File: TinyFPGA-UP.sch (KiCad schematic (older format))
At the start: 35 parts, among them J1 Conn_01x14, J2 Conn_01x14, J3 USB_B_Micro, J4 Conn_02x08_Odd_Even, J5 Conn_02x03_Odd_Even, SW1 SW_Push, U1 iCE40-UP5K-SG48, U2 MIC5504-3.3, U3 DSC6001CI2A, U4 MIC5365-1.2, U5 AT25SF081

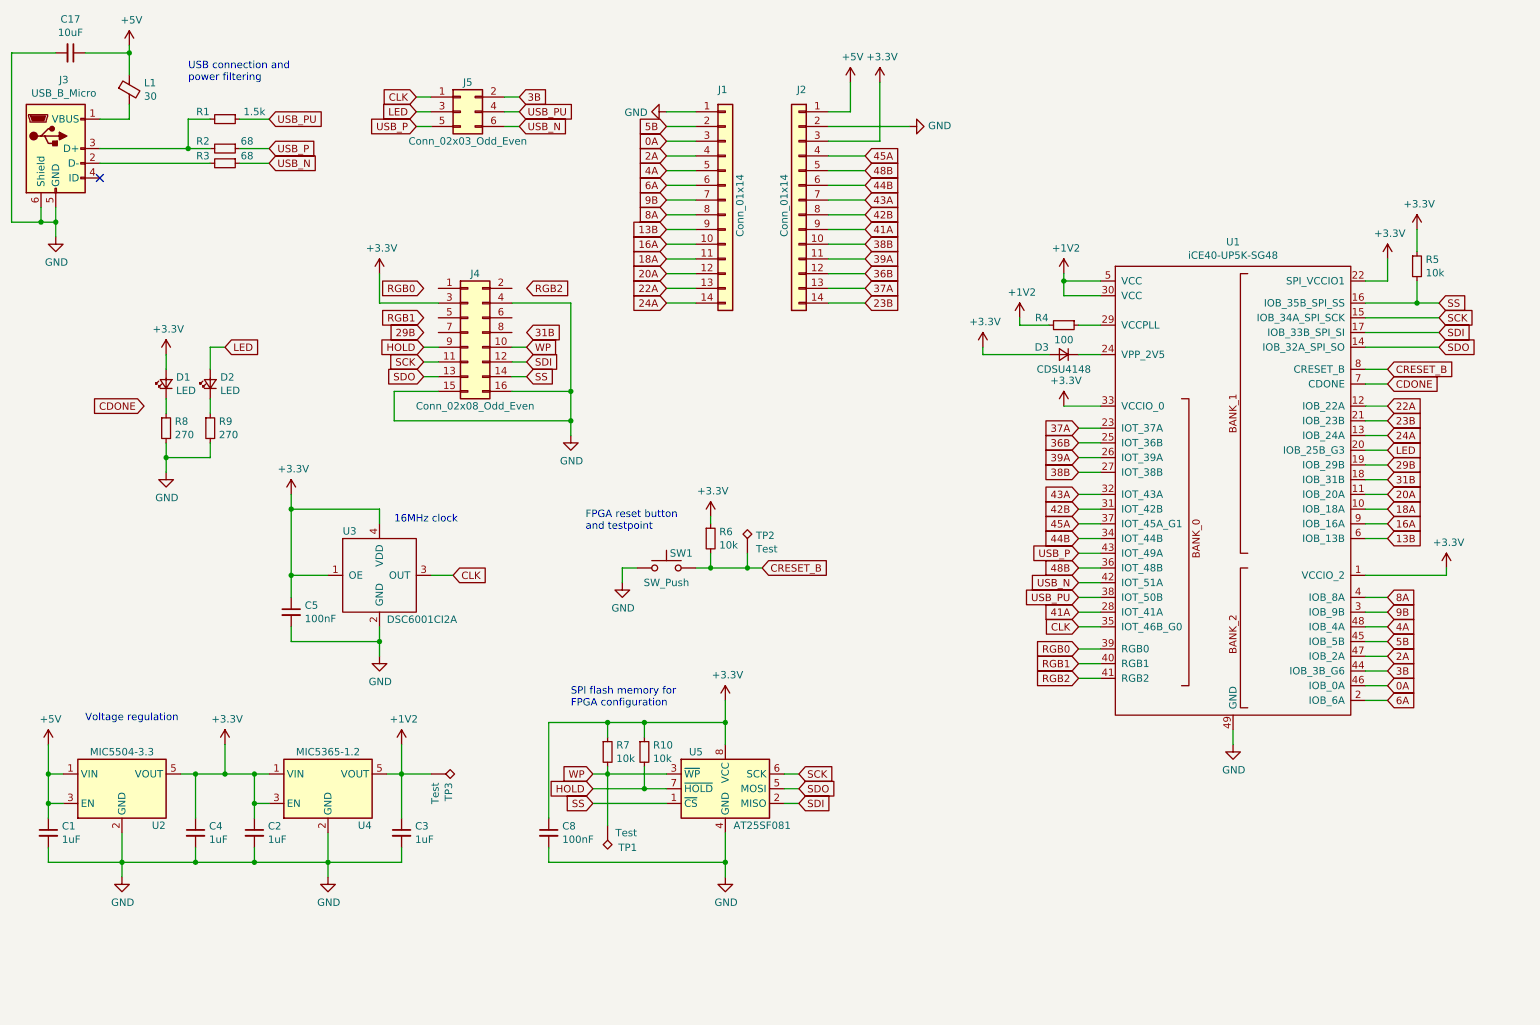
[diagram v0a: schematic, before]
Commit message: Update routing
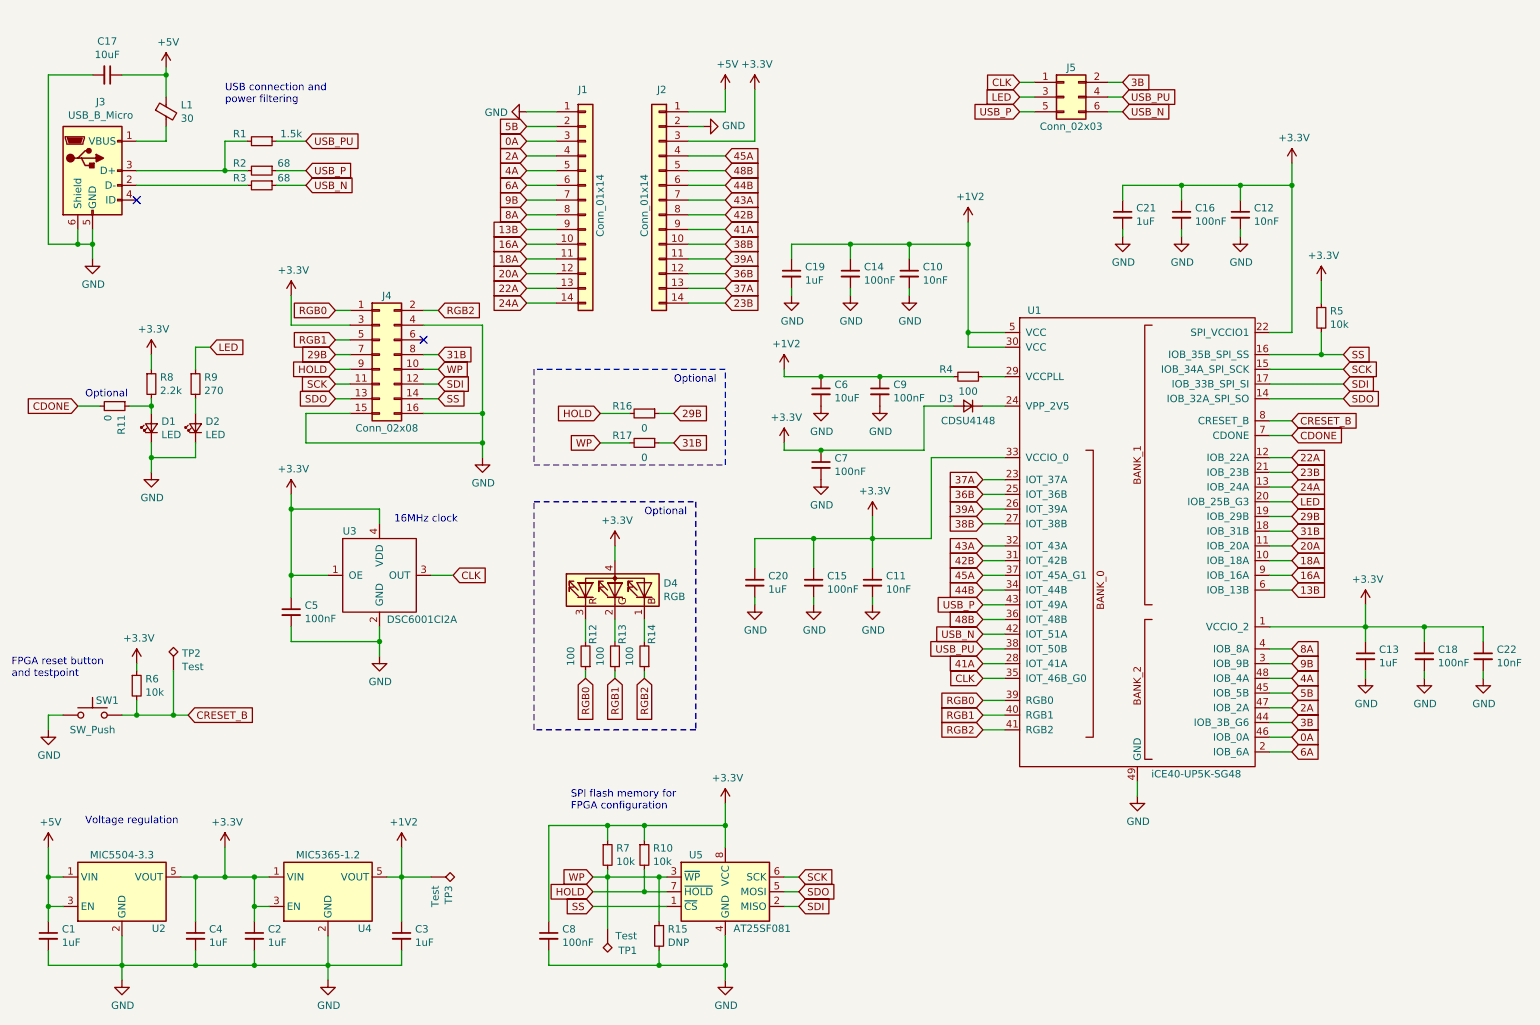
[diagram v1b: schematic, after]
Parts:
- added C10, C11, C12, C22: 10nF, Capacitor_SMD:C_0402_1005Metric, symbol Device:C_Small
- added C13, C19, C20, C21: 1uF, Capacitor_SMD:C_0402_1005Metric, symbol Device:C_Small
- added C14, C15, C16, C18, C7, C9: 100nF, Capacitor_SMD:C_0402_1005Metric, symbol Device:C_Small
- added C6: 10uF, Capacitor_SMD:C_0402_1005Metric, symbol Device:C_Small
- added D4: RGB, DRA818:LTST-C19HE1WT, symbol Device:LED_BGRA
- added R11, R16, R17: 0, Resistor_SMD:R_0402_1005Metric, symbol Device:R_Small
- added R12, R13, R14: 100, Resistor_SMD:R_0402_1005Metric, symbol Device:R_Small
- added R15: DNP, Resistor_SMD:R_0402_1005Metric, symbol Device:R_Small
- J4: value Conn_02x08_Odd_Even -> Conn_02x08
- J5: value Conn_02x03_Odd_Even -> Conn_02x03
- R8: value 270 -> 2.2k
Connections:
- net +1V2: now also C10.1, C14.1, C19.1, C6.1, C9.1
- net +3V3: now also R8.1, C11.1, C12.1, C13.1, C15.1, C16.1, C18.1, C20.1, C21.1, C22.1, C7.1, D4.4 (A); no longer D1.2 (A)
- net 29B: now also J4.7 (Pin_7), R16.1
- net 31B: now also J4.8 (Pin_8), R17.1
- net CDONE: now also R11.2
- net GND: now also D1.1 (K), D2.1 (K), C10.2, C11.2, C12.2, C13.2, C14.2, C15.2, C16.2, C18.2, C19.2, C20.2, C21.2, C22.2, C6.2, C7.2, C9.2, R15.2; no longer R8.2, R9.2
- net HOLD: now also R16.2
- net LED: now also R9.1; no longer D2.2 (A)
- net RGB0: now also J4.1 (Pin_1), R12.1
- net RGB1: now also J4.5 (Pin_5), R13.1
- net RGB2: now also J4.2 (Pin_2), R14.1
- net WP: now also R15.1, R17.2
- new net: D1.2 (A), R11.1, R8.2
- new net: D4.1 (BK), R14.2
- new net: D4.2 (GK), R13.2
- new net: D4.3 (RK), R12.2
- new net: D2.2 (A), R9.2
- no-connect marks 1 -> 2
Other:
- note added: "Optional"
- moved on the sheet: C1, C17, C2, C3, C4, C8, D1, D2, D3, J1, J2, J3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
